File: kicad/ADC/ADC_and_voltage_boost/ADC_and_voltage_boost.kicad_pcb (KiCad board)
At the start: 2 copper layers, 29.7 x 43.4 mm, 12 parts, among them J1 Screw_Terminal_01x04, J2 Screw_Terminal_01x04, U3 MOUDLE-SEEEDUINO-XIAO-ESP32C3, U4 MAX1032BEUG_

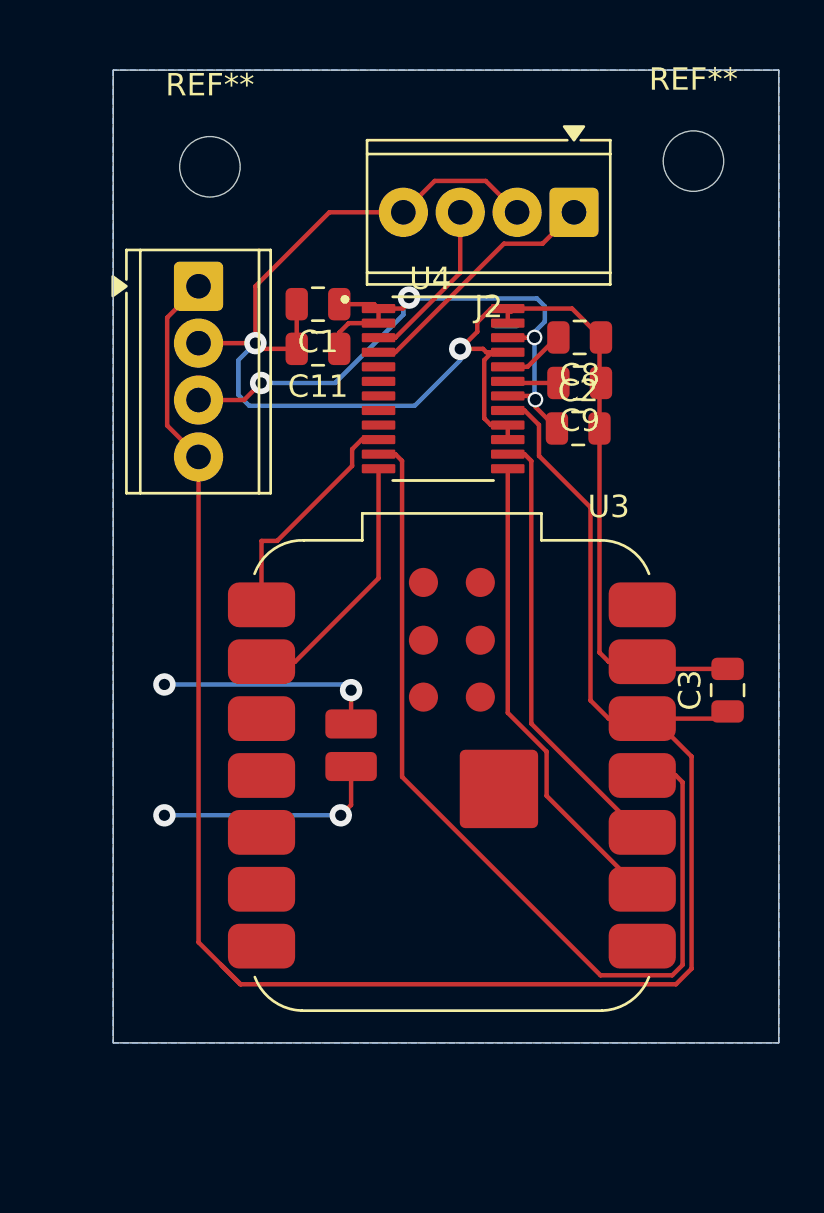
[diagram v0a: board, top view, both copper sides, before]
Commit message: added ino file
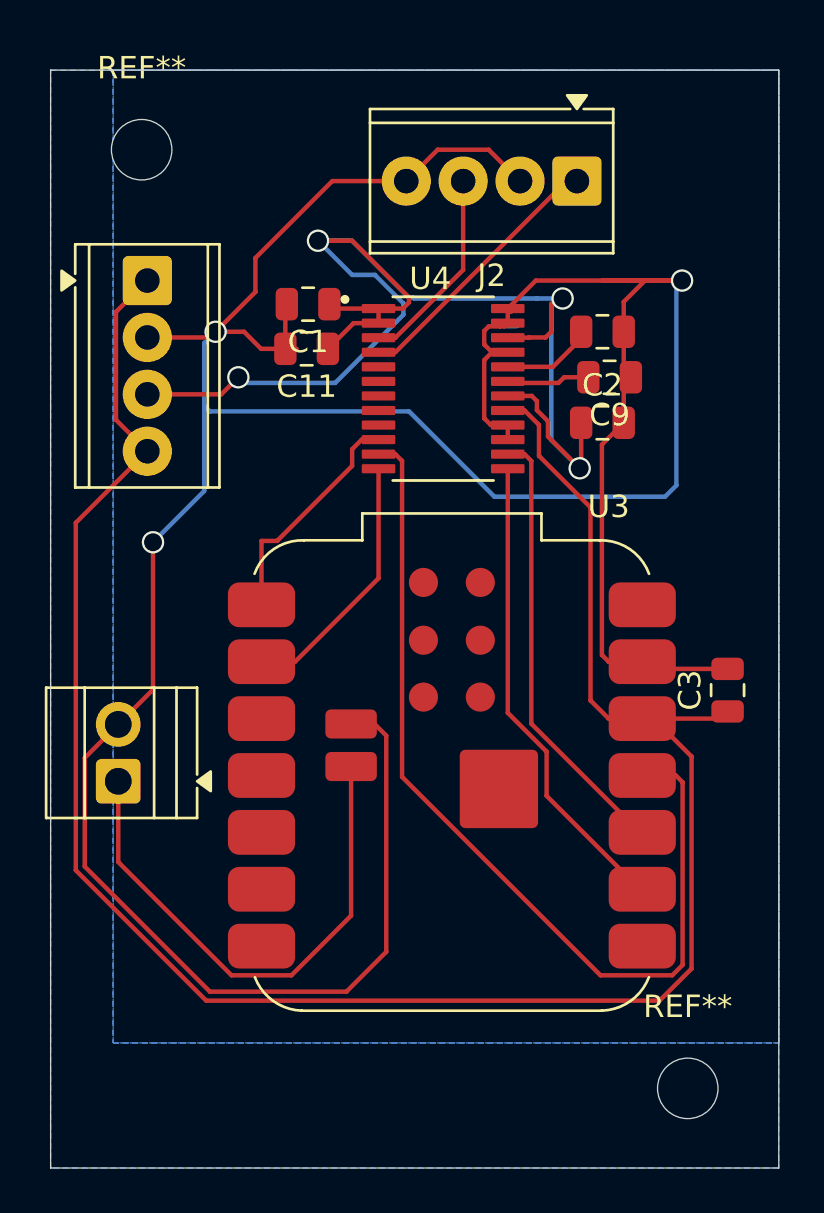
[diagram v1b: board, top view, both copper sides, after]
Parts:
- added REF**: TerminalBlock_Xinya_XY308-2.54-2P_1x02_P2.54mm_Horizontal, TerminalBlock:TerminalBlock_Xinya_XY308-2.54-2P_1x02_P2.54mm_Horizontal, F.Cu at (135.1, 114.3)
- moved REF** 41.4 mm to (160.5, 128.0)
- moved REF** 3.14 mm to (136.1, 86.1)
- moved J1 2.30 mm to (136.4, 91.9)
- moved J2 1.40 mm to (155.6, 87.5)
- moved C9 1.36 mm to (157.0, 96.3)
- moved C2 1.11 mm to (156.7, 98.3)
- moved C8 1.05 mm to (156.7, 94.2)
- moved C11 0.51 mm to (143.5, 95.0)
- moved C1 0.44 mm to (143.6, 93.0)
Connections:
- U3 pad 16: (no net) -> +3.3V
- U3 pad 17: (no net) -> GND
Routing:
- net GND: track 75.1 -> 161.4 mm, vias 2 -> 3
- net +5V: track 32.8 -> 62.7 mm
- net +3.3V: track 88.2 -> 116.6 mm
- net (no net): track 20.2 -> 0.00 mm, vias 4 -> 0
- net Net-(J2-Pin_3): track 7.55 -> 9.00 mm
- net Net-(U4-REF): track 2.74 -> 4.10 mm
- net Net-(U4-REFCAP): track 2.29 -> 3.41 mm
- net Net-(J2-Pin_1): track 11.3 -> 12.0 mm
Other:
- board size 29.7 x 43.4 mm -> 32.5 x 49 mm
- board text removed: "Screw_Terminal_01x04"
